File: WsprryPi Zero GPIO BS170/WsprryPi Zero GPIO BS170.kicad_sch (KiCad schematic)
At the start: 26 parts, among them J11 Socket_2x20_P2.54mm, J12 Conn_01x03, J51 SMA_Adafruit_1865, J52 J81/J82 LPF sockets, Q41 BS170, SW11 SKRPANE010, U11 Raspberry Pi 40-pin HAT inter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, U21 TPS22918DBVR

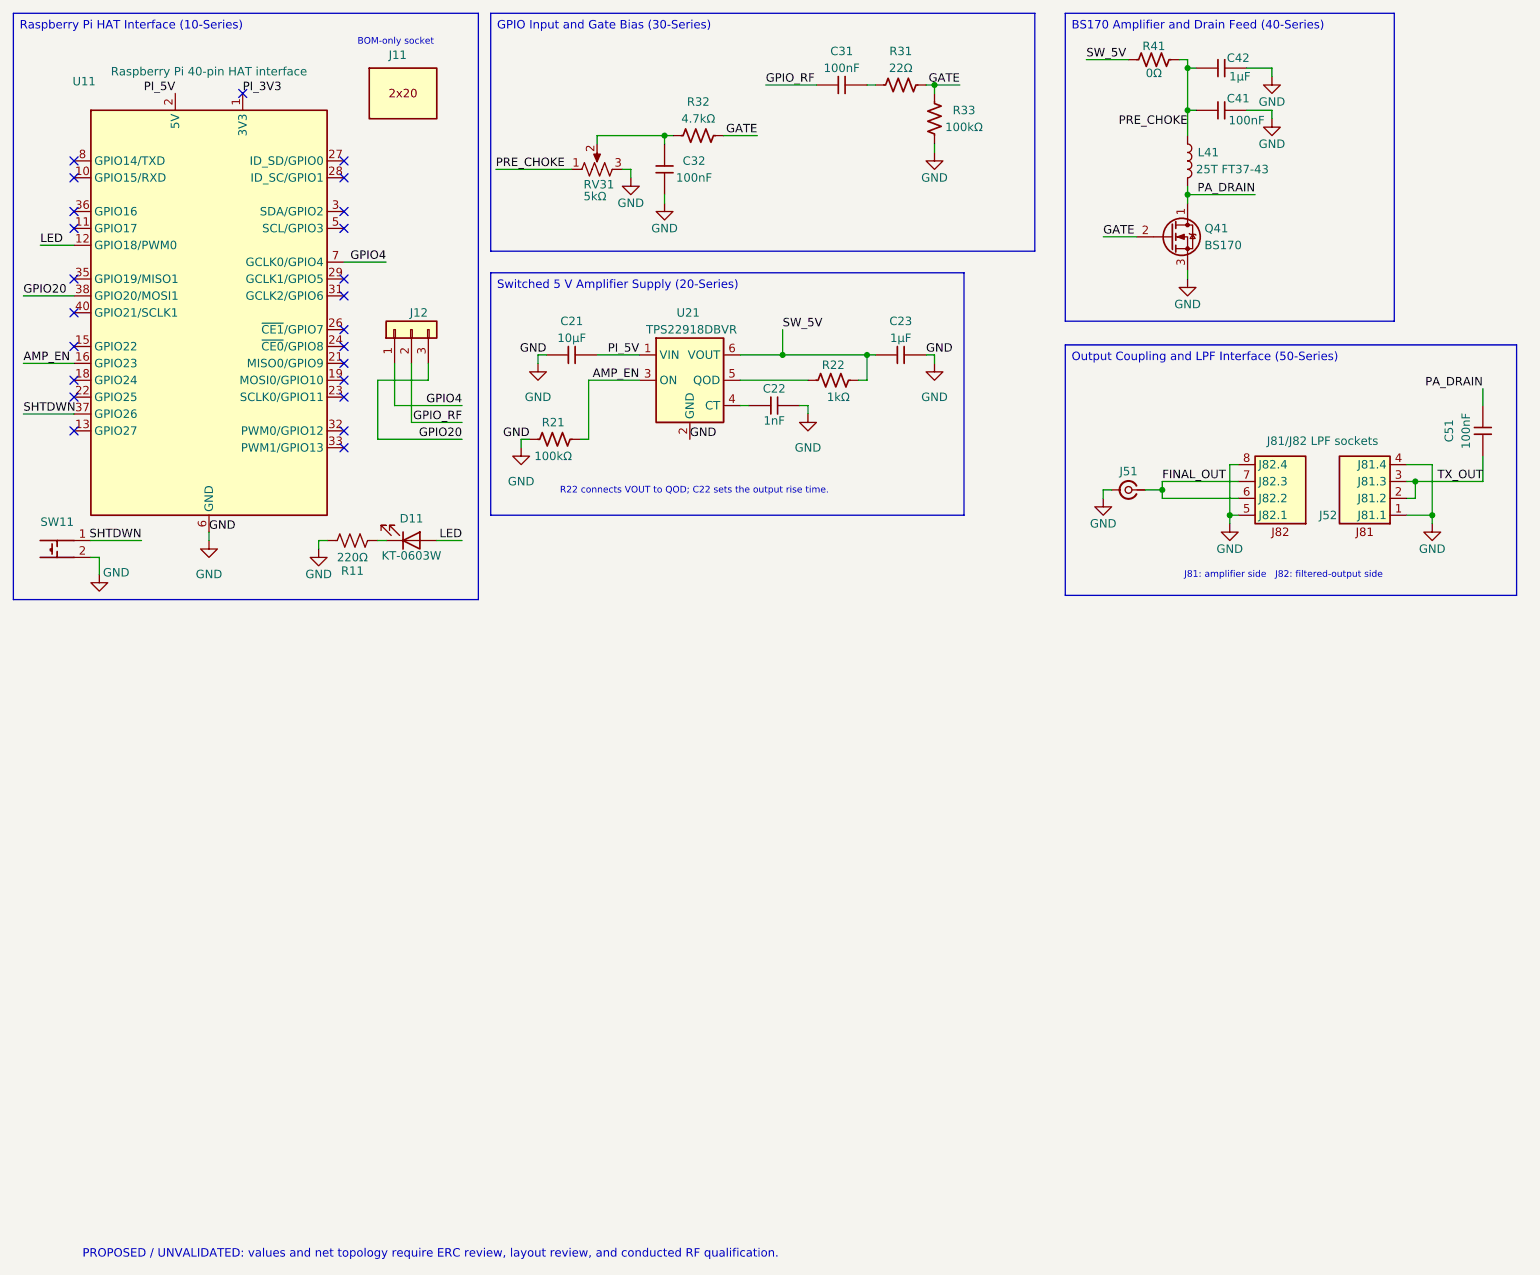
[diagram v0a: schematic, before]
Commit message: File rename and cleanup
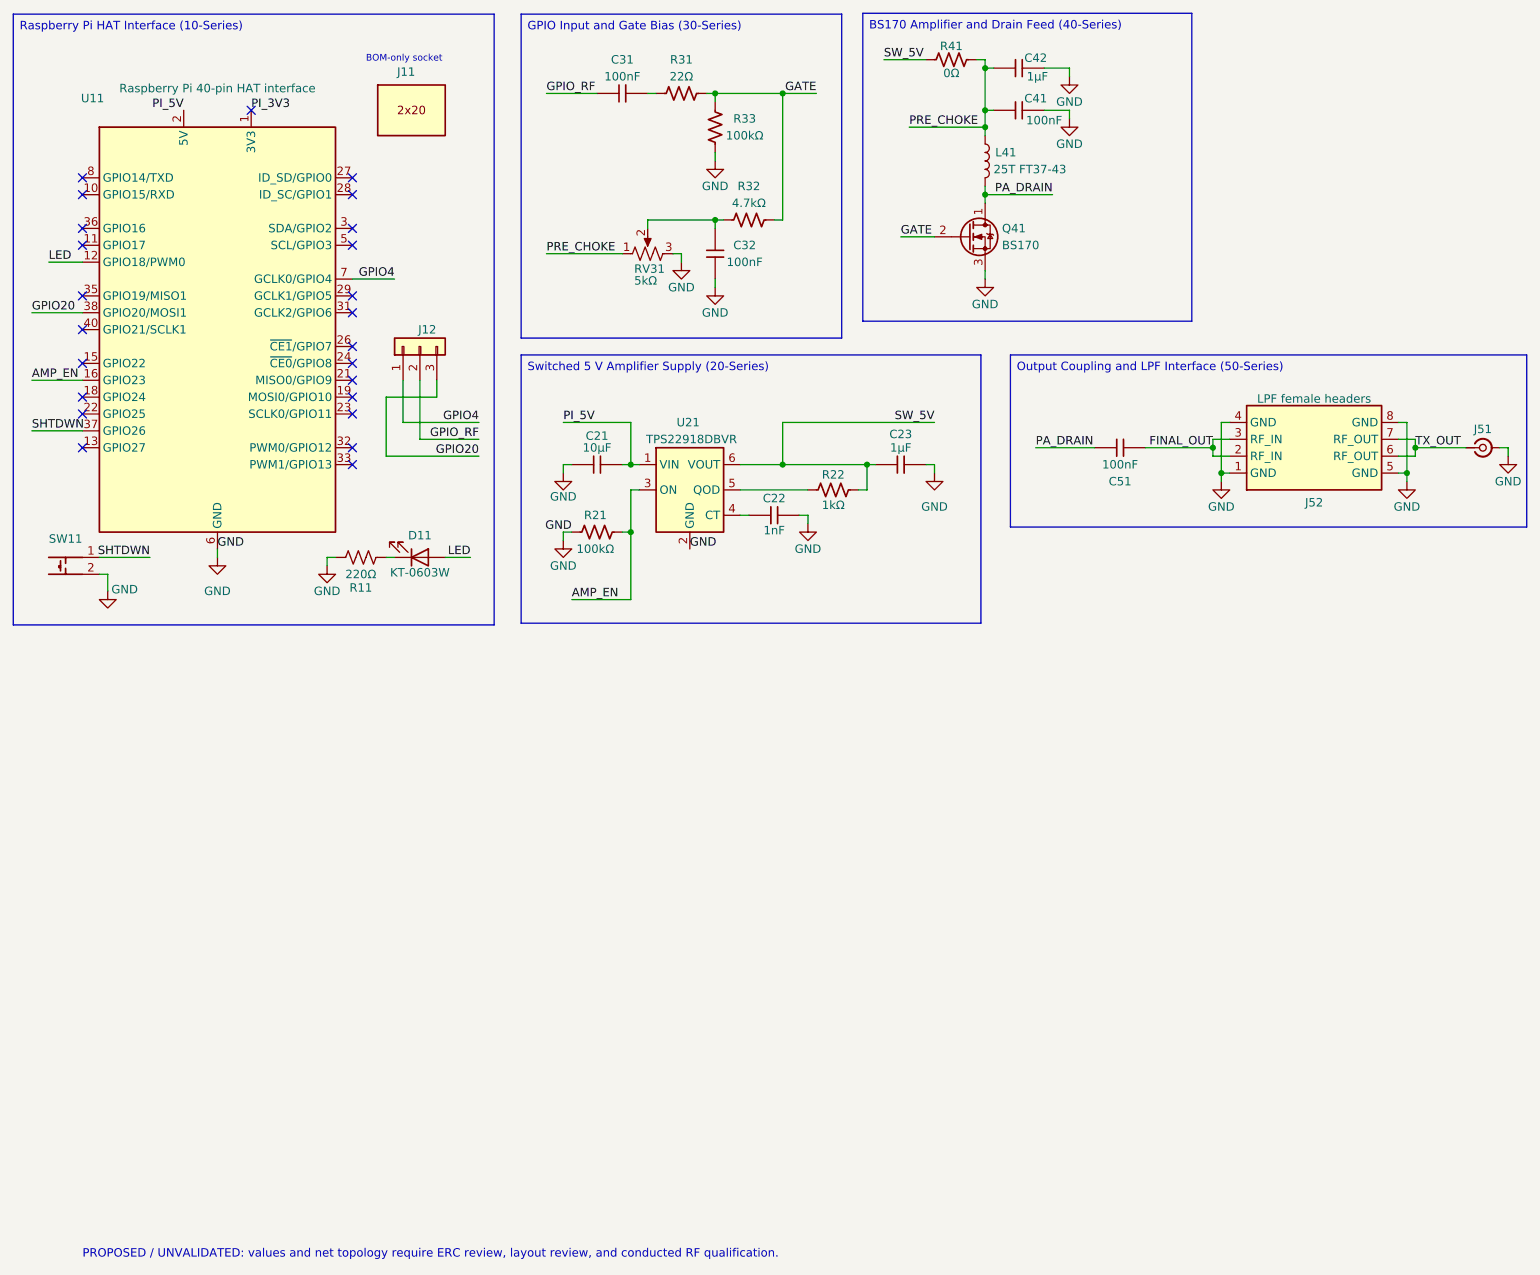
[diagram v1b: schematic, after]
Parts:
- J52: value J81/J82 LPF sockets -> LPF female headers; footprint wsprrypi-zero-gpio-bs170:Dual_PinSocket_1x04_P2.54mm_J81_J82 -> wsprrypi-zero-gpio-bs170:LPF_HeaderPair_Female_2x1x04_P2.54mm_S33.02mm; symbol wsprrypi-zero-gpio-bs170:Dual_PinSocket_1x04_P2.54mm_J81_J82 -> wsprrypi-zero-gpio-bs170:LPF_HeaderPair_Female_2x1x04_P2.54mm_S33.02mm
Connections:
- net FINAL_OUT: now also C51.2, J52.2 (RF_IN), J52.3 (RF_IN); no longer J51.1 (In), J52.6 (J82.2), J52.7 (J82.3)
- net PA_DRAIN: now also C51.1; no longer C51.2
- net TX_OUT: now also J51.1 (In), J52.6 (RF_OUT), J52.7 (RF_OUT); no longer C51.1, J52.2 (J81.2), J52.3 (J81.3)
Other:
- note removed: "J81: amplifier side J82: filtered-output side"
- note removed: "R22 connects VOUT to QOD; C22 sets the output rise time."
- moved on the sheet: C21, C22, C23, C31, C32, C41, C42, C51, D11, J11, J12, J51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
